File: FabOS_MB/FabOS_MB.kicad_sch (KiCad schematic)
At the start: 2 parts, among them U1 STM32F407VETx

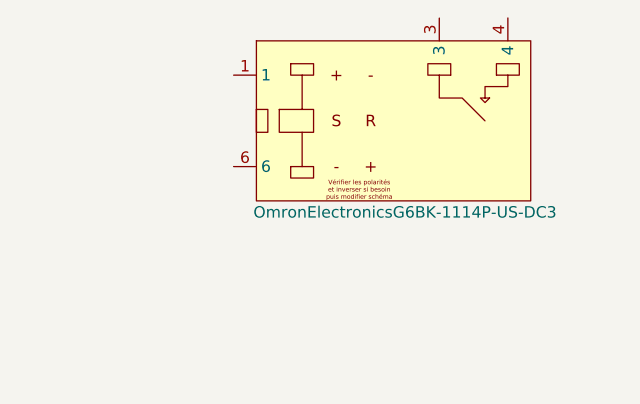
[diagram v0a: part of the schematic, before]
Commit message: MàJ Kicad
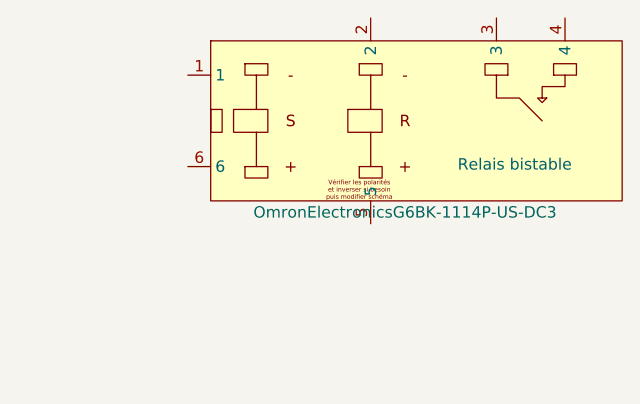
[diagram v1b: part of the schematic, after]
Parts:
- OmronElectronicsG6BK-1114P-US-DC3: LCSC (none) -> C1563013; MPN (none) -> G6BK-1114P-US-DC3
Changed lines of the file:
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@@
 		(on_board yes)
 		(dnp no)
-		(fields_autoplaced yes)
 		(property "Reference" "OmronElectronicsG6BK-1114P-US-DC3"
 			(at 129.54 43.18 0)
@@
 			)
 		)
-		(property "Datasheet" ""
+		(property "Datasheet" "https://www.lcsc.com/datasheet/lcsc_datasheet_2211282100_Omron-Electronics-G6BK-1114P-US-DC3_C1563013.pdf"
 			(at 107.95 33.02 0)
 			(effects
@@
 			)
 		)
-		(property "Description" ""
-			(at 107.95 33.02 0)
+		(property "Description" "Relais bistable"
+			(at 141.732 37.846 0)
+			(effects
+				(font
+					(size 1.27 1.27)
+				)
+			)
+		)
+		(property "MPN" " G6BK-1114P-US-DC3"
+			(at 128.27 33.02 0)
+			(effects
+				(font
+					(size 1.27 1.27)
+				)
+				(hide yes)
+			)
+		)
+		(property "LCSC" " C1563013"
+			(at 128.27 33.02 0)
 			(effects
 				(font
@@
 		(pin "6"
 		)
+		(pin "5"
+		)
+		(pin "2"
+		)
 		(instances
